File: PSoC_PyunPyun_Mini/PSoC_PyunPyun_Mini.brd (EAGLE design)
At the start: 100 x 80 mm, 33 parts, among them IC1 LM358N, IC2 LM358N

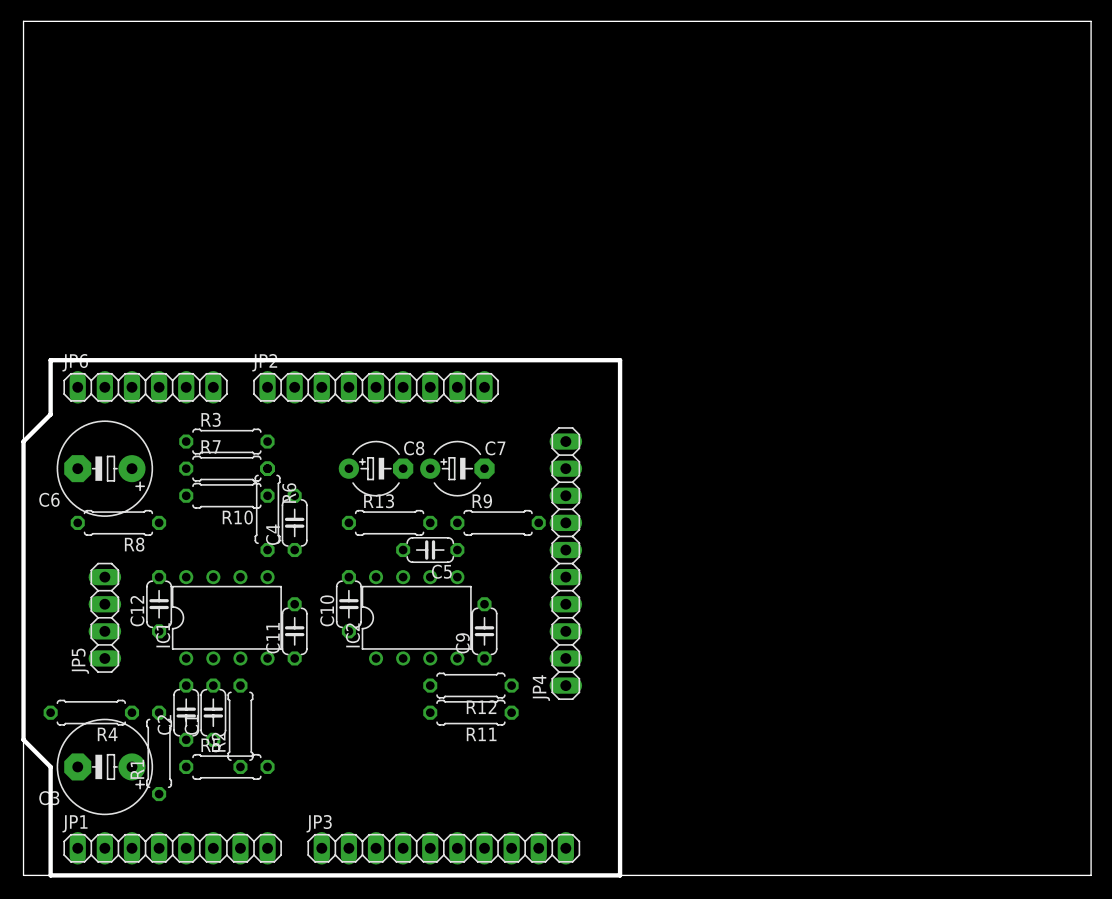
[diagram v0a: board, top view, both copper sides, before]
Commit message: PSoC Pyun Pyunの基板図を作成
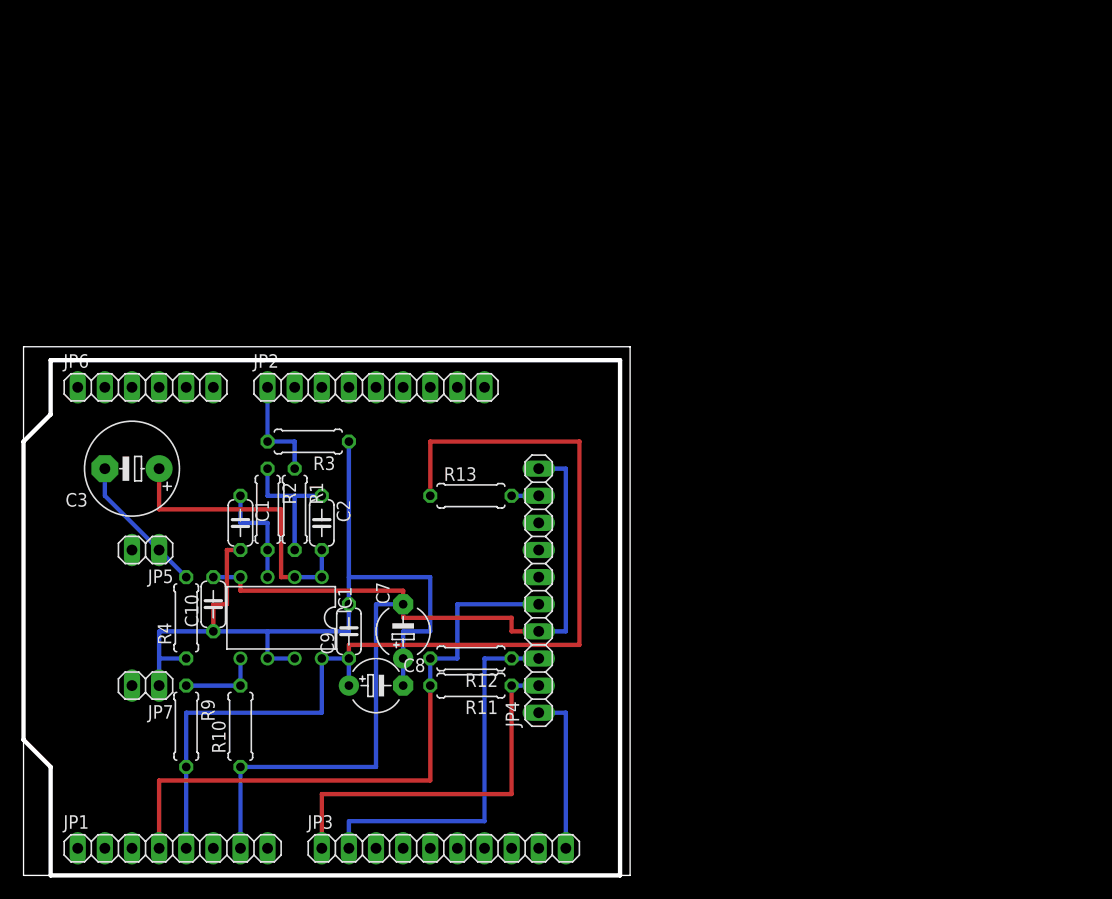
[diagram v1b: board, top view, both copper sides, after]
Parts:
- removed C11, C12: 0.1u, rcl:C050-024X044
- removed C4, C5: 0.001uF, rcl:C050-024X044
- removed C6: 220uF, rcl:E5-8,5
- removed IC2: LM358N, linear:DIL08
- removed R5, R6, R8: 10k, rcl:0207/7
- removed R7: 2.2k, rcl:0207/7
- added JP7: RCA_GND, pinhead:1X02
- JP5: value 3.5mm Jack -> RCA_HOT; device pinhead:1X04 -> pinhead:1X02
- moved R9 34.9 mm to (15.2, 14.0), turned to 270 degrees
- moved C3 28.1 mm to (10.2, 38.1)
- moved R1 26.2 mm to (25.4, 34.3), turned to 270 degrees
- moved C2 21.8 mm to (27.9, 33.0), turned to 270 degrees
- moved R10 21.6 mm to (20.3, 14.0), turned to 90 degrees
- moved R2 20.5 mm to (22.9, 34.3), turned to 270 degrees
- moved C8 20.3 mm to (33.0, 17.8)
- moved C1 18.0 mm to (20.3, 33.0), turned to 270 degrees
- moved C7 16.1 mm to (35.6, 22.9), turned to 90 degrees
- moved C10 12.7 mm to (17.8, 25.4)
- moved C9 12.7 mm to (30.5, 22.9)
- moved R4 12.6 mm to (15.2, 24.1), turned to 90 degrees
- moved R13 8.03 mm to (41.9, 35.6)
- moved R3 7.62 mm to (26.7, 40.6), turned to 180 degrees
- moved JP5 7.41 mm to (11.4, 30.5), turned to 180 degrees
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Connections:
- removed net N$11: C4.1, IC1.5, R6.2
- removed net N$12: C5.2, C6.+, IC1.6, IC1.7
- removed net N$14: C6.-, JP5.4, R8.2
- removed net N$9: C5.1, R5.2, R6.1
- removed net V+: IC1.8, IC2.8
- removed net V-: IC1.4, IC2.4
- net +5V: now also IC1.8; no longer C10.1, C11.1, C12.1
- net AGND: now also C10.1, C9.2, IC1.6, IC1.7, JP7.1; no longer C4.2, IC2.1, IC2.2, IC2.6, IC2.7, JP5.2, R7.1, R8.1
- net GND: now also IC1.4; no longer C11.2, C12.2, C9.2
- net IDAC7: no longer R5.1, R7.2
- net N$8: now also IC1.5; no longer IC2.3, IC2.5
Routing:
- net +5V: track 0.00 -> 96.5 mm
- net GND: track 0.00 -> 94.0 mm
- net AGND: track 0.00 -> 78.7 mm
- net +3.3V: track 0.00 -> 58.4 mm
- net SCL: track 0.00 -> 35.6 mm
- net SDA: track 0.00 -> 35.6 mm
- net N$4: track 0.00 -> 27.9 mm
- net RST: track 0.00 -> 15.2 mm
- net N$7: track 0.00 -> 13.3 mm
- net N$1: track 0.00 -> 12.7 mm
- net N$3: track 0.00 -> 10.2 mm
- net IDAC8: track 0.00 -> 10.2 mm
- net N$8: track 0.00 -> 7.62 mm
- net N$5: track 0.00 -> 2.54 mm
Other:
- board size 100 x 80 mm -> 56.8 x 49.5 mm
